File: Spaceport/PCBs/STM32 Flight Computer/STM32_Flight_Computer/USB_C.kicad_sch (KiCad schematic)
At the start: 2 parts, among them J1 USB4105-GF-A-060, U6 USBLC6-2P6

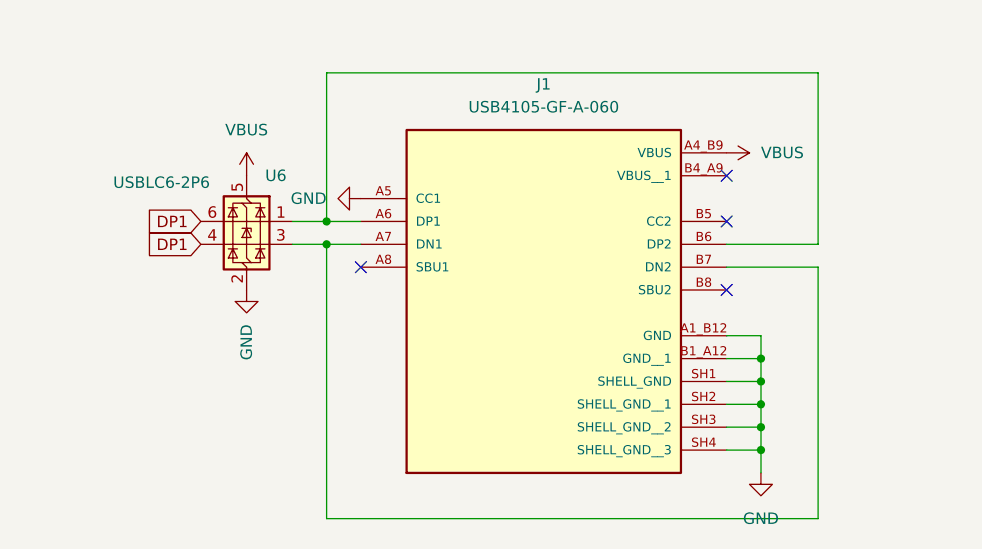
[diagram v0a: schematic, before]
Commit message: Push after Schematic Review 5/5
- Updated STM32 symbol
- Configured I2C busses
- Updated DC caps to 100nF
- TODO add power system things
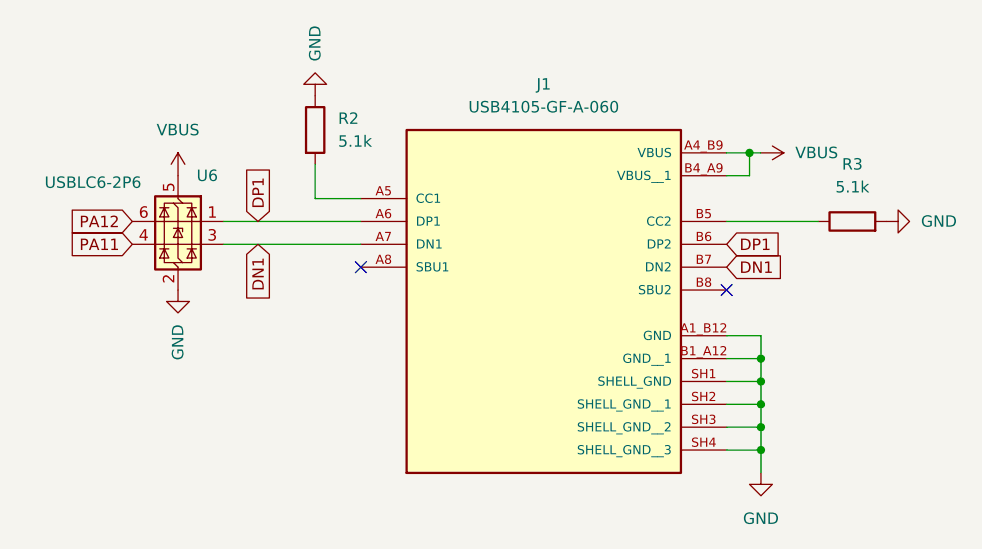
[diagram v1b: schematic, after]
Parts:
- added R2, R3: 5.1k, symbol Device:R
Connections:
- net DP1: now also J1.A6 (DP1), J1.B6 (DP2), U6.1 (I/O1); no longer U6.4 (I/O2), U6.6 (I/O1)
- net GND: now also R2.1, R3.2; no longer J1.A5 (CC1)
- net VBUS: now also J1.B4_A9 (VBUS__1)
- net DN1: now reaches J1.A7 (DN1), J1.B7 (DN2), U6.3 (I/O2)
- net at J1.B5 (CC2): now also R3.1
- new net: J1.A5 (CC1), R2.2
- new net PA11: U6.4 (I/O2)
- new net PA12: U6.6 (I/O1)
- no-connect marks 4 -> 2
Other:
- moved on the sheet: U6
